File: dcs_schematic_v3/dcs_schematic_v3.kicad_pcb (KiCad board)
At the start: 4 copper layers, 68 parts, among them J1 691137710002, J2 1728307, Q1 IRLZ44N, U2 LM311DR, U3 LM2917N/NOPB, U4 HEF4030BT, U5 CDBW140-G

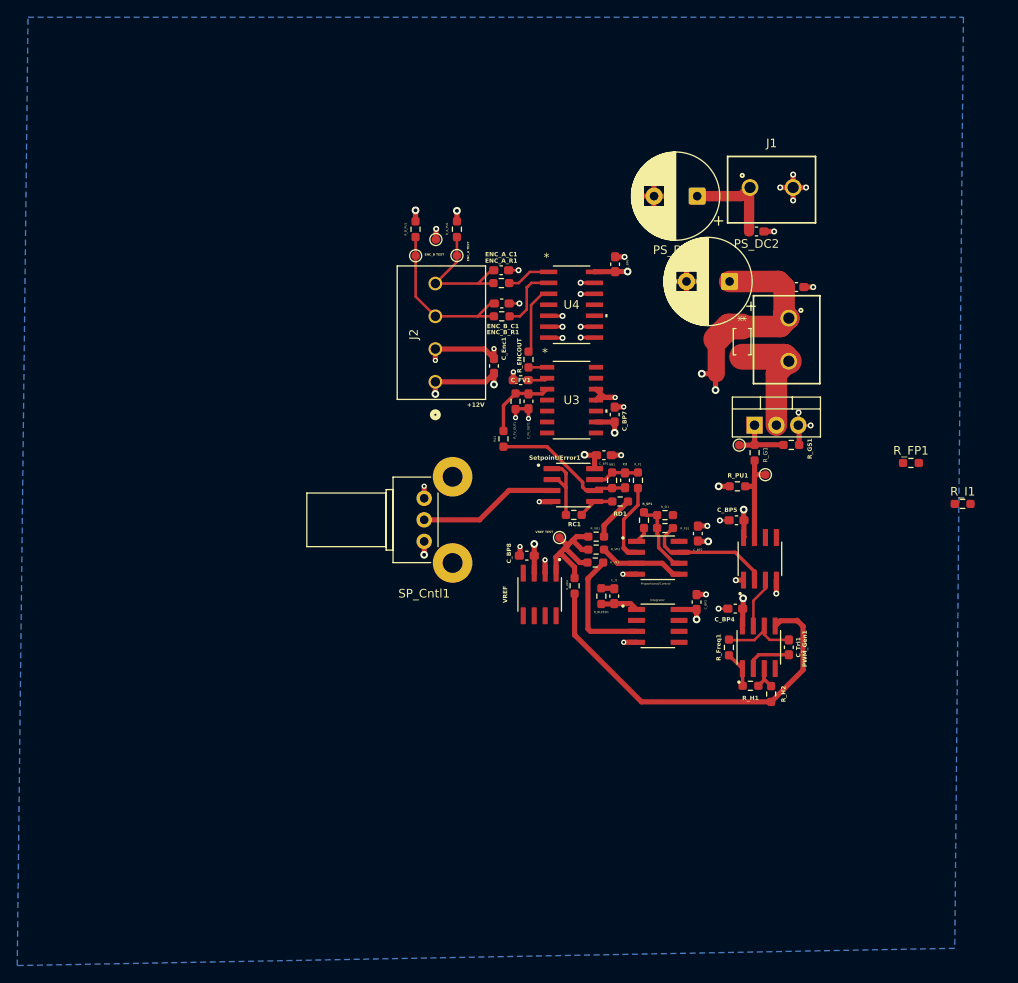
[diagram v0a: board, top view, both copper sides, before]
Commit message: changed diode again. updated datasheets, models, etc.
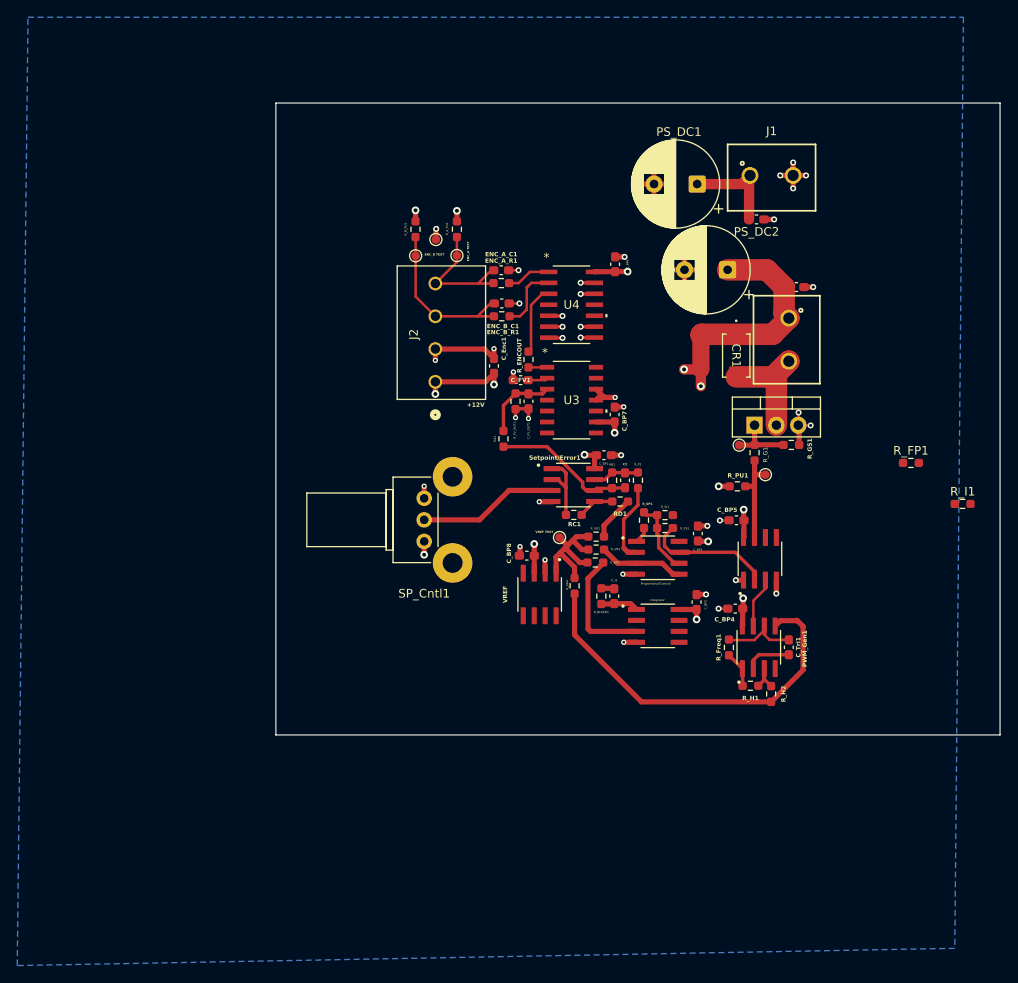
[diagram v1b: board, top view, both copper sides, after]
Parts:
- removed U5: CDBW140-G, CapstoneLibrary:CDBW_Diode
- added CR1: SK34A-LTP, CapstoneLibrary:SK32A-LTP_Diode, F.Cu at (154.9, 81.5)
- moved NT1 1.85 mm to (150.8, 81.1)
- moved J1 1.40 mm to (159.0, 60.6)
- moved PS_DC1 1.40 mm to (150.4, 61.6)
- moved PS_DC2 1.40 mm to (157.2, 65.7)
- moved C_M+1 1.37 mm to (153.9, 71.5)
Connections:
- R_SP1 pad 1: Net-(Proportional/Control1--INB) -> /V_P
- R_SP1 pad 2: /V_P -> Net-(Proportional/Control1--INB)
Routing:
- net /M+: track 19.9 -> 22.2 mm
- net /M-: track 13.7 -> 14.9 mm
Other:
- board outline added: 84 x 73.3 mm
